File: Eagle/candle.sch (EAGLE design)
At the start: 17 parts, among them J1 AVR_SPI_PRG_6NS, U1 Tiny85-20-SMT

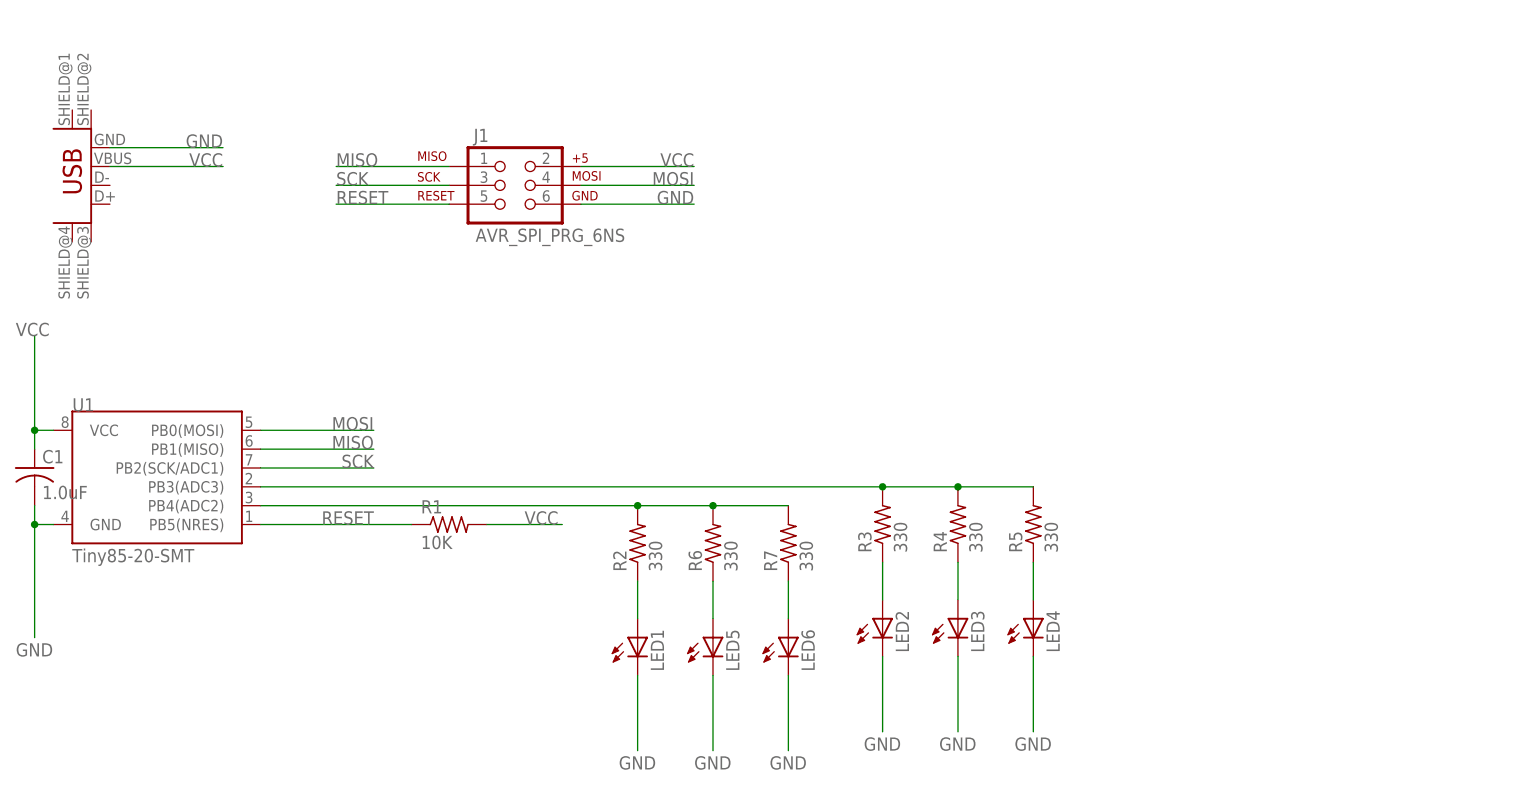
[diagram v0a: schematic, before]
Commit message: Combine branches into one branch.
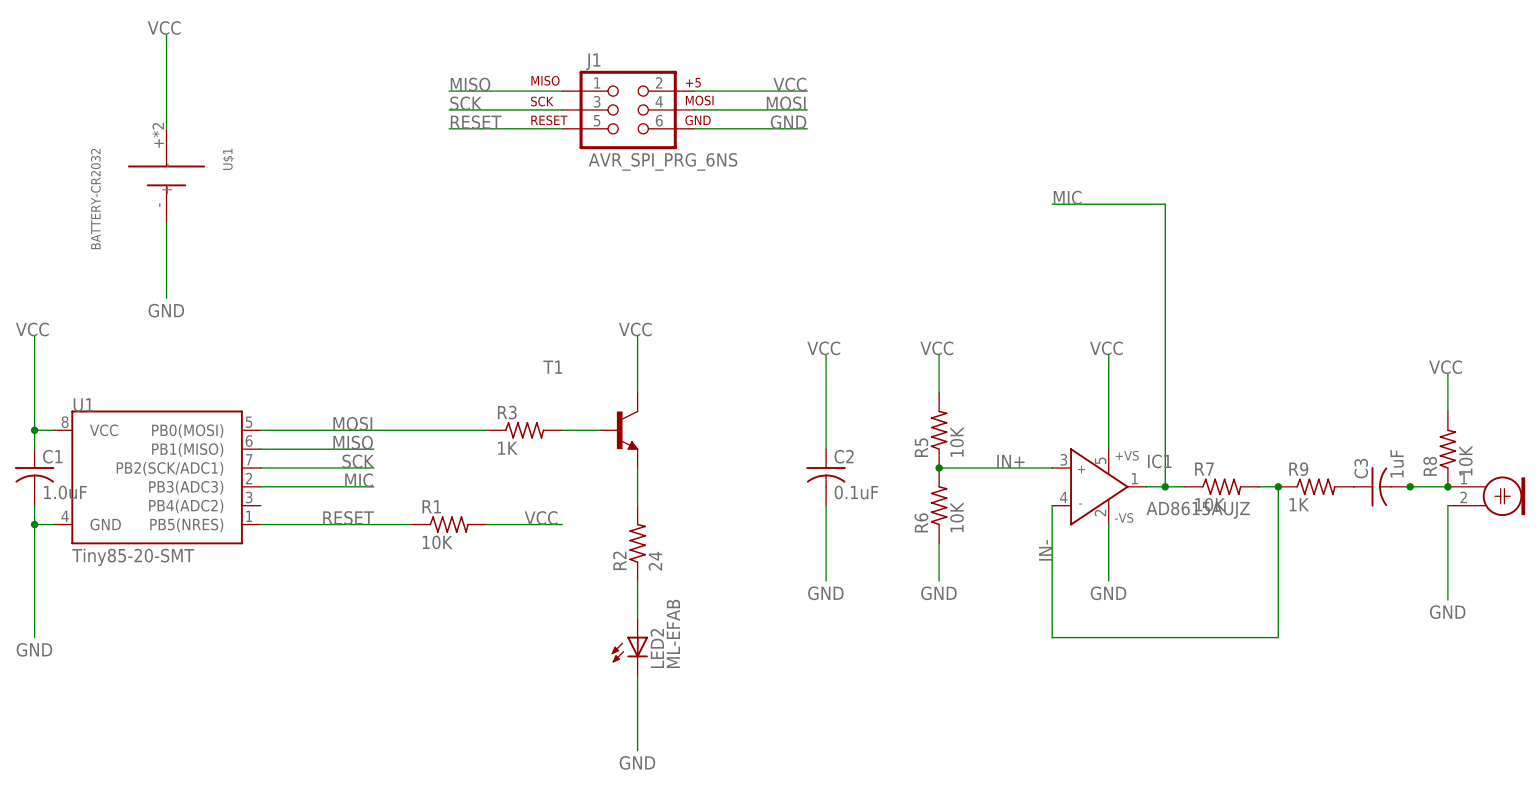
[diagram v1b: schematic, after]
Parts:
- removed JP1: USB_MINIB, fab:USB_MINIB
- removed LED1, LED3, LED4, LED5, LED6: (no value), led:LEDSMT1206
- removed R4: 330, rcl:R-US_R1206
- added C2: 0.1uF, rcl:C-USC1206
- added C3: 1uF, rcl:C-USC1206
- added IC1: AD8615AUJZ, analog-devices:AD8614RJ
- added M1: ELECTRETTH, LED Light:ELECTRETTH
- added R8: 10K, rcl:R-US_R1206
- added R9: 1K, rcl:R-US_R1206
- added T1: (no value), transistor:MMBT3904LT1-NPN-SOT23-BEC
- added U$1: BATTERY-CR2032, LED Light:BATTERY-CR2032
- LED2: value (none) -> ML-EFAB; device led:LEDSMT1206 -> LED Light:ML-EFAB
- R2: value 330 -> 24
- R3: value 330 -> 1K
- R5, R6, R7: value 330 -> 10K
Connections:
- removed net N$5: LED6.A, R7.1
- removed net N$7: LED3.A, R4.1
- removed net N$8: LED4.A, R5.1
- new net IN+: IC1.IN+, R5.1, R6.2
- new net IN-: IC1.IN-, R7.2, R9.1
- new net MIC: IC1.OUT, R7.1, U1.PB3(ADC3)
- net GND: now also C2.2, IC1.-VS, LED2G$1.C@1, M1.2, R6.1, U$1.-; no longer JP1.GND, LED1.C, LED2.C, LED3.C, LED4.C, LED5.C, LED6.C
- net MOSI: now also R3.1
- net N$1: now also T1.E; no longer R6.2, R7.2, U1.PB4(ADC2)
- net N$2: now also T1.B; no longer R4.2, R5.2, U1.PB3(ADC3)
- net N$3: now also LED2G$1.A@1; no longer LED1.A
- net N$4: now also C3.2, M1.1, R8.1; no longer LED2.A, R3.1
- net N$6: now also C3.1, R9.2; no longer LED5.A, R6.1
- net VCC: now also C2.1, IC1.+VS, R5.2, R8.2, T1.C, U$1.+; no longer JP1.VBUS
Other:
- moved on the sheet: J1, R3, R5, R6, R7
